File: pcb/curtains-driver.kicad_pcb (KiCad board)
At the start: 2 copper layers, 71 x 29.7 mm, 25 parts, among them J1 Barrel_Jack, J2 UART, J3 Motor, SW1 Reed_NC, SW2 Reed_NC, SW3 UP, SW4 DOWN, SW5 FLASH, U1 ESP-12F, U2 LM1117-3.3, U3 ULN2003

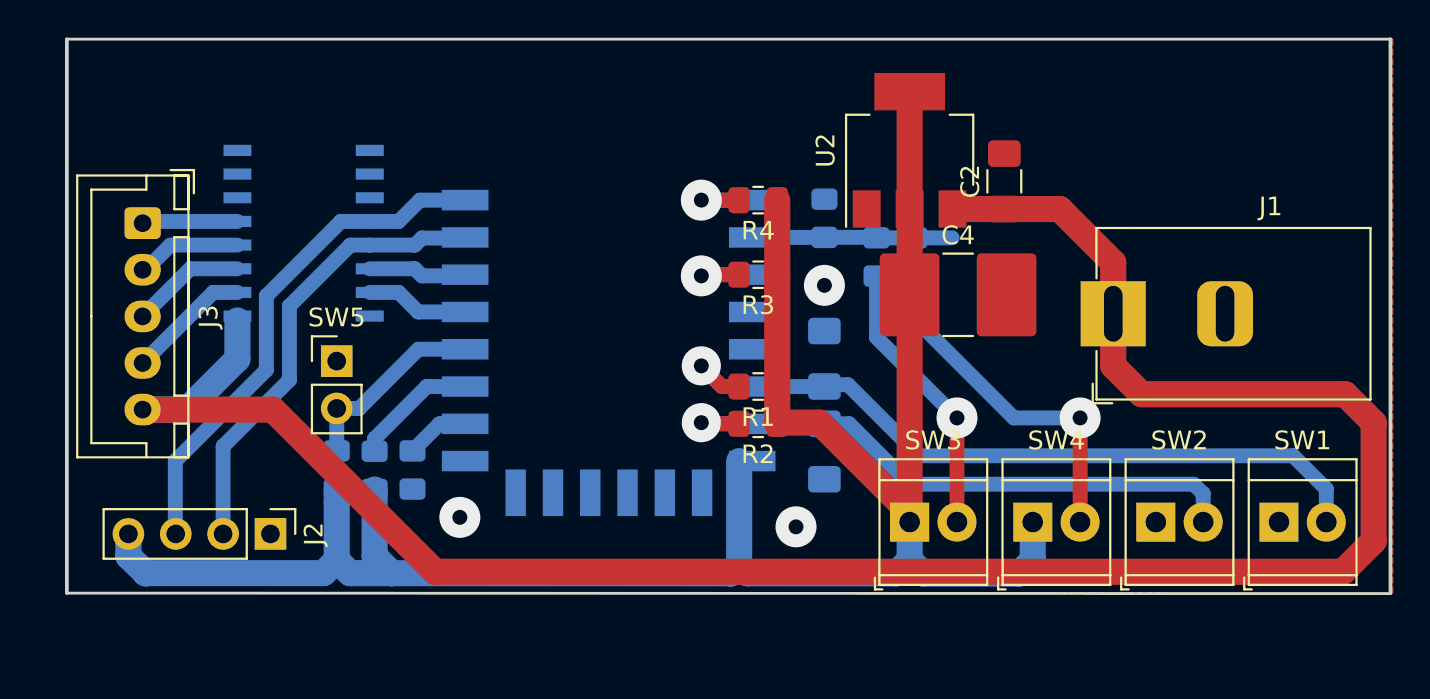
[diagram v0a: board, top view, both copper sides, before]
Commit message: Refactor Circuit
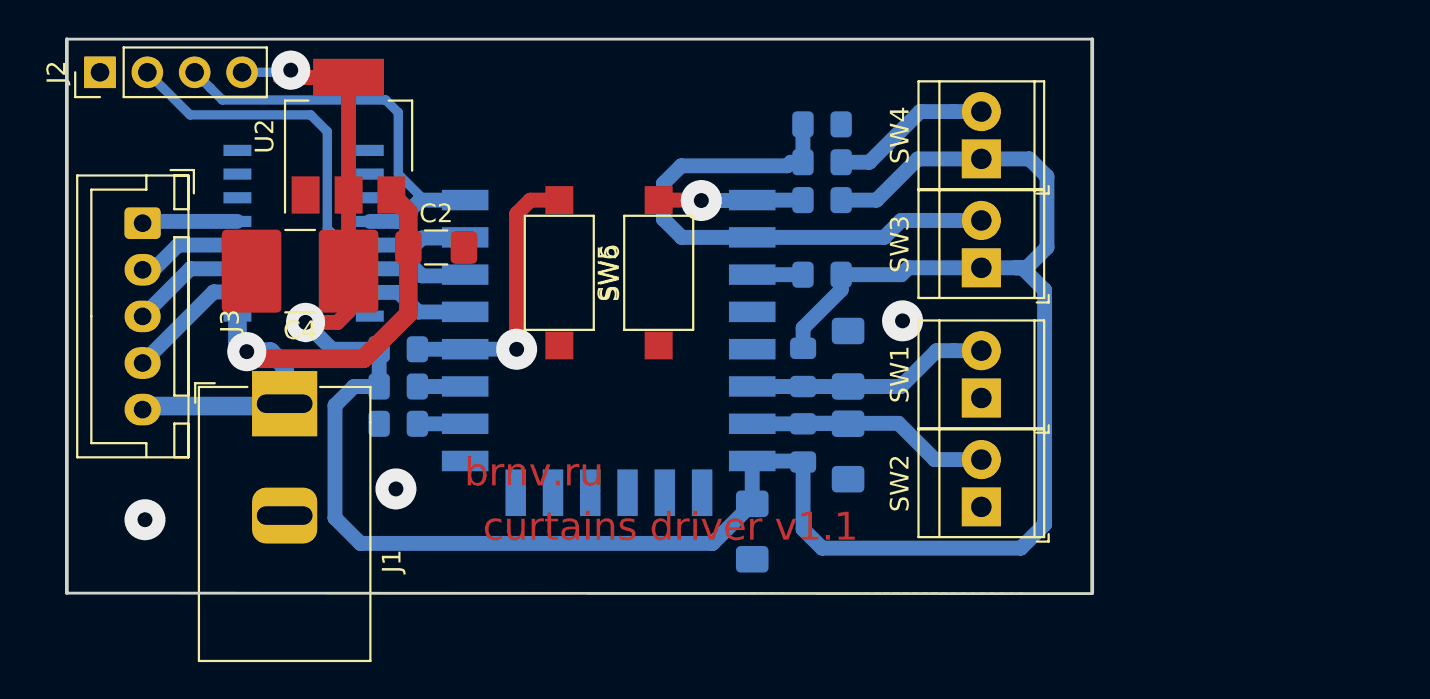
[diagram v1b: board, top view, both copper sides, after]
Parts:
- removed R9: 10K, Resistor_SMD:R_0805_2012Metric_Pad1.15x1.40mm_HandSolder
- added C5: 0.1uF, Capacitor_SMD:C_1206_3216Metric_Pad1.42x1.75mm_HandSolder, B.Cu at (115.8, 90.2)
- added SW6: RESET, Button_Switch_SMD:SW_SPST_CK_RS282G05A3, F.Cu at (110.7, 76.3)
- R1, R2, R3, R4: value 10K -> R; moved to B.Cu
- R5, R6, R7: value 10K -> R
- R8: value 5K1 -> 56K
- SW5: footprint Connector_PinHeader_2.54mm:PinHeader_1x02_P2.54mm_Vertical -> Button_Switch_SMD:SW_SPST_CK_RS282G05A3
- moved J1 44.7 mm to (90.7, 83.3), turned to 90 degrees
- moved C4 35.3 mm to (91.5, 76.2), turned to 180 degrees
- moved C2 30.7 mm to (98.8, 74.9), turned to 0 degrees
- moved U2 30.1 mm to (94.1, 69.0)
- moved J2 26.4 mm to (80.8, 65.5), turned to 90 degrees
- moved SW4 19.7 mm to (128.1, 70.2), turned to 90 degrees
- moved SW1 17.3 mm to (128.1, 83.0), turned to 90 degrees
- moved SW3 14.2 mm to (128.1, 76.0), turned to 90 degrees
- moved R4 13.2 mm to (118.5, 85.4), turned to 270 degrees
- moved SW5 12.8 mm to (105.4, 76.3), turned to 270 degrees
- moved R1 10.6 mm to (119.5, 72.4), turned to 0 degrees
- moved SW2 9.40 mm to (128.1, 88.8), turned to 90 degrees
- moved R2 8.70 mm to (119.5, 76.4), turned to 0 degrees
- moved R7 6.52 mm to (96.8, 80.4), turned to 0 degrees
- moved R8 5.86 mm to (119.5, 70.4), turned to 0 degrees
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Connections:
- C4 pad 1: +3V3 -> VCC
- J2 pad 4: +3V3 -> VCC
- R1 pad 1: +3V3 -> Net-(R1-Pad1)
- R1 pad 2: Net-(C1-Pad1) -> VCC
- R2 pad 1: +3V3 -> Net-(R2-Pad1)
- R2 pad 2: Net-(C3-Pad1) -> VCC
- R3 pad 1: +3V3 -> Net-(C1-Pad1)
- R3 pad 2: Net-(R3-Pad2) -> VCC
- R4 pad 1: +3V3 -> Net-(C3-Pad1)
- R4 pad 2: Net-(R4-Pad2) -> VCC
- R5 pad 1: +3V3 -> Earth
- R6 pad 1: +3V3 -> VCC
- R7 pad 1: Earth -> VCC
- SW3 pad 1: +3V3 -> VCC
- SW3 pad 2: Net-(R8-Pad2) -> ADC
- SW4 pad 1: +3V3 -> VCC
- SW4 pad 2: Net-(R9-Pad2) -> Net-(R8-Pad2)
- SW5 pad 1: Earth -> Net-(R7-Pad2)
- SW5 pad 2: Net-(R5-Pad2) -> Earth
- U1 pad 1: Net-(R4-Pad2) -> Net-(R1-Pad1)
- U1 pad 10: Net-(R7-Pad2) -> Net-(R5-Pad2)
- U1 pad 12: Net-(R5-Pad2) -> Net-(R7-Pad2)
- U1 pad 3: Net-(R3-Pad2) -> Net-(R2-Pad1)
- U1 pad 8: +3V3 -> VCC
- U2 pad 2: +3V3 -> VCC
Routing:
- net VCC: track 0.00 -> 132.2 mm, vias 0 -> 2
- net +3V3: track 114.7 -> 0.00 mm
- net +5V: track 115.8 -> 30.8 mm, vias 0 -> 1
- net Net-(C1-Pad1): track 40.6 -> 13.8 mm, vias 1 -> 0
- net Net-(R9-Pad2): track 19.0 -> 0.00 mm, vias 1 -> 0
- net ADC: track 11.4 -> 29.6 mm
- net Net-(C3-Pad1): track 32.1 -> 15.7 mm, vias 1 -> 0
- net Net-(R7-Pad2): track 4.13 -> 15.2 mm, vias 0 -> 1
- net Net-(R5-Pad2): track 11.2 -> 3.26 mm
- net Net-(R1-Pad1): track 0.00 -> 7.76 mm, vias 0 -> 1
- net Net-(R8-Pad2): track 15.0 -> 8.65 mm, vias 1 -> 0
- net Net-(R6-Pad2): track 7.39 -> 3.26 mm
- net Net-(R3-Pad2): track 4.11 -> 0.00 mm, vias 1 -> 0
- net Net-(R4-Pad2): track 4.05 -> 0.00 mm, vias 1 -> 0
- net Net-(R2-Pad1): track 0.00 -> 3.42 mm
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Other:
- board size 71 x 29.7 mm -> 55 x 29.7 mm
- net class Resistor Array added: clearance 0.3, trace_width 0.6, via_dia 0.8, via_drill 0.4
- board text added: "brnv.ru"
- board text added: "curtains driver v1.1"
